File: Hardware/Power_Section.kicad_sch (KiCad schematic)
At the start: 39 parts, among them IC1 TPS54202HDDCR, Q1 SI2347DS-T1-GE3, U1 TLV743P, U2 TLV743P, U3 TLV743P, U4 TLV743P

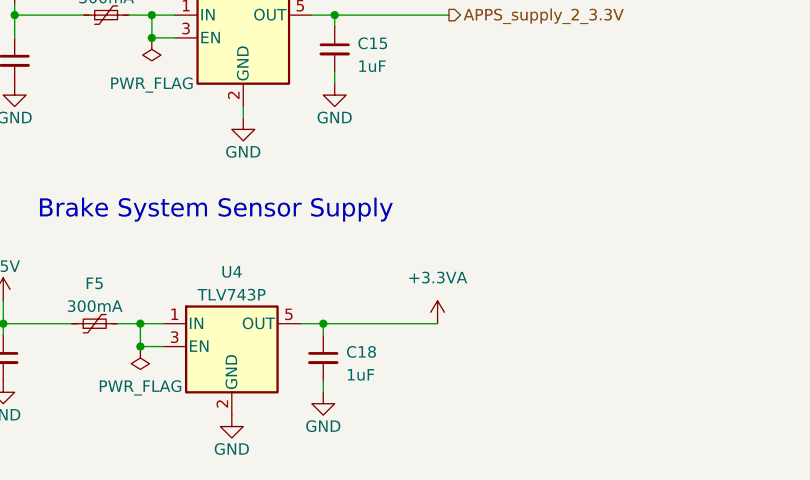
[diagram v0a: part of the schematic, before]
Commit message: Changes in CAN section
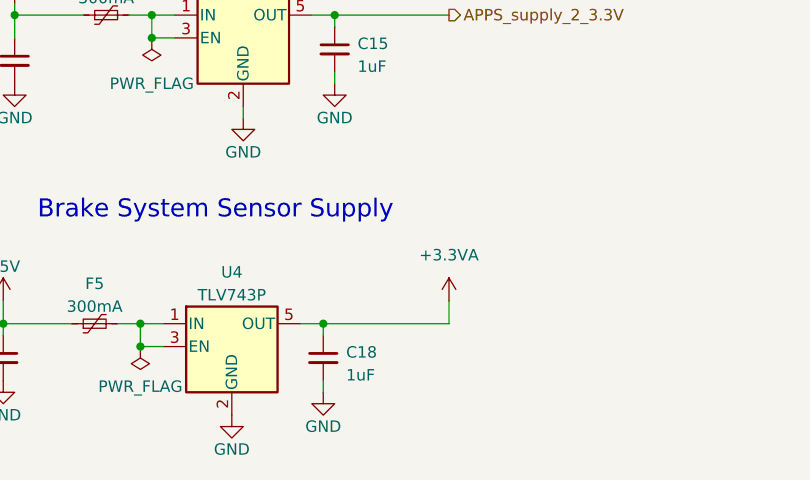
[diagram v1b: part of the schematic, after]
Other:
- title: (none) -> FrontBox
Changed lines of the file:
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@@
 	(generator_version "9.0")
 	(paper "A4")
+	(title_block
+		(title "FrontBox")
+	)
 	(text "APPS Potentiometer 2 supply"
 		(exclude_from_sim no)
@@
 	)
 	(junction
-		(at 64.77 172.72)
-		(diameter 0)
-		(color 0 0 0 0)
-	)
-	(junction
 		(at 245.11 59.69)
 		(diameter 0)
@@
 	)
 	(junction
+		(at 64.77 172.72)
+		(diameter 0)
+		(color 0 0 0 0)
+	)
+	(junction
 		(at 218.44 46.99)
 		(diameter 0)
@@
 	(wire
 		(pts
-			(xy 64.77 172.72) (xy 77.47 172.72)
-		)
-		(stroke
-			(width 0)
-			(type default)
-		)
-	)
-	(wire
-		(pts
 			(xy 25.4 72.39) (xy 25.4 73.66)
 		)
@@
 	(wire
 		(pts
+			(xy 64.77 172.72) (xy 78.74 172.72)
+		)
+		(stroke
+			(width 0)
+			(type default)
+		)
+	)
+	(wire
+		(pts
 			(xy 25.4 78.74) (xy 25.4 80.01)
 		)
@@
 	(wire
 		(pts
+			(xy 78.74 172.72) (xy 78.74 170.18)
+		)
+		(stroke
+			(width 0)
+			(type default)
+		)
+	)
+	(wire
+		(pts
 			(xy 245.11 46.99) (xy 255.27 46.99)
 		)
@@
 	(symbol
 		(lib_id "power:+3.3VA")
-		(at 77.47 172.72 0)
+		(at 78.74 170.18 0)
 		(unit 1)
 		(exclude_from_sim no)
@@
 		(dnp no)
 		(property "Reference" "#PWR036"
-			(at 77.47 176.53 0)
+			(at 78.74 173.99 0)
 			(effects
 				(font
@@
 		)
 		(property "Value" "+3.3VA"
-			(at 77.47 167.64 0)
+			(at 78.74 165.1 0)
 			(effects
 				(font
@@
 		)
 		(property "Footprint" ""
-			(at 77.47 172.72 0)
+			(at 78.74 170.18 0)
 			(effects
 				(font
@@
 		)
 		(property "Datasheet" ""
-			(at 77.47 172.72 0)
+			(at 78.74 170.18 0)
 			(effects
 				(font
@@
 		)
 		(property "Description" ""
-			(at 77.47 172.72 0)
+			(at 78.74 170.18 0)
 			(effects
 				(font

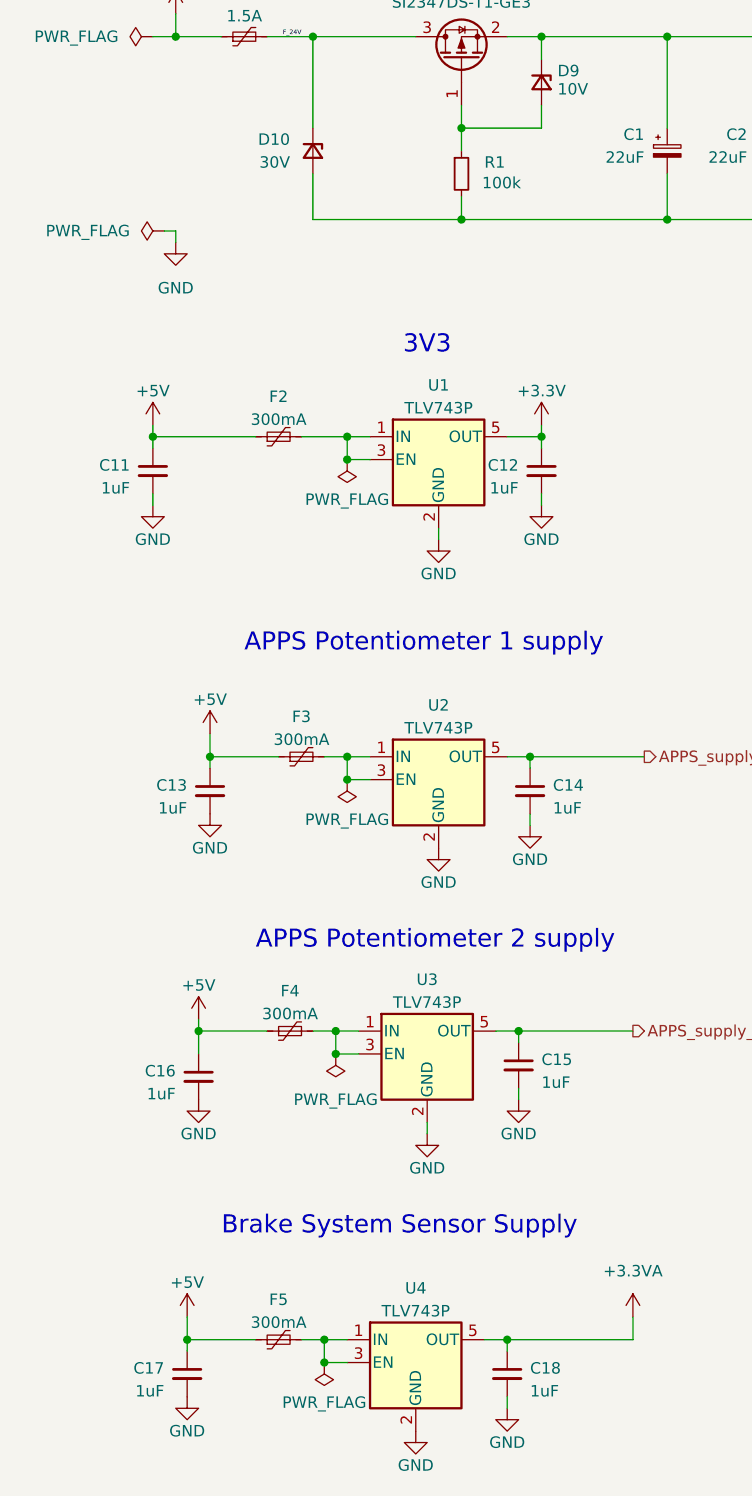
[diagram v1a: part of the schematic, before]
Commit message: BOM update
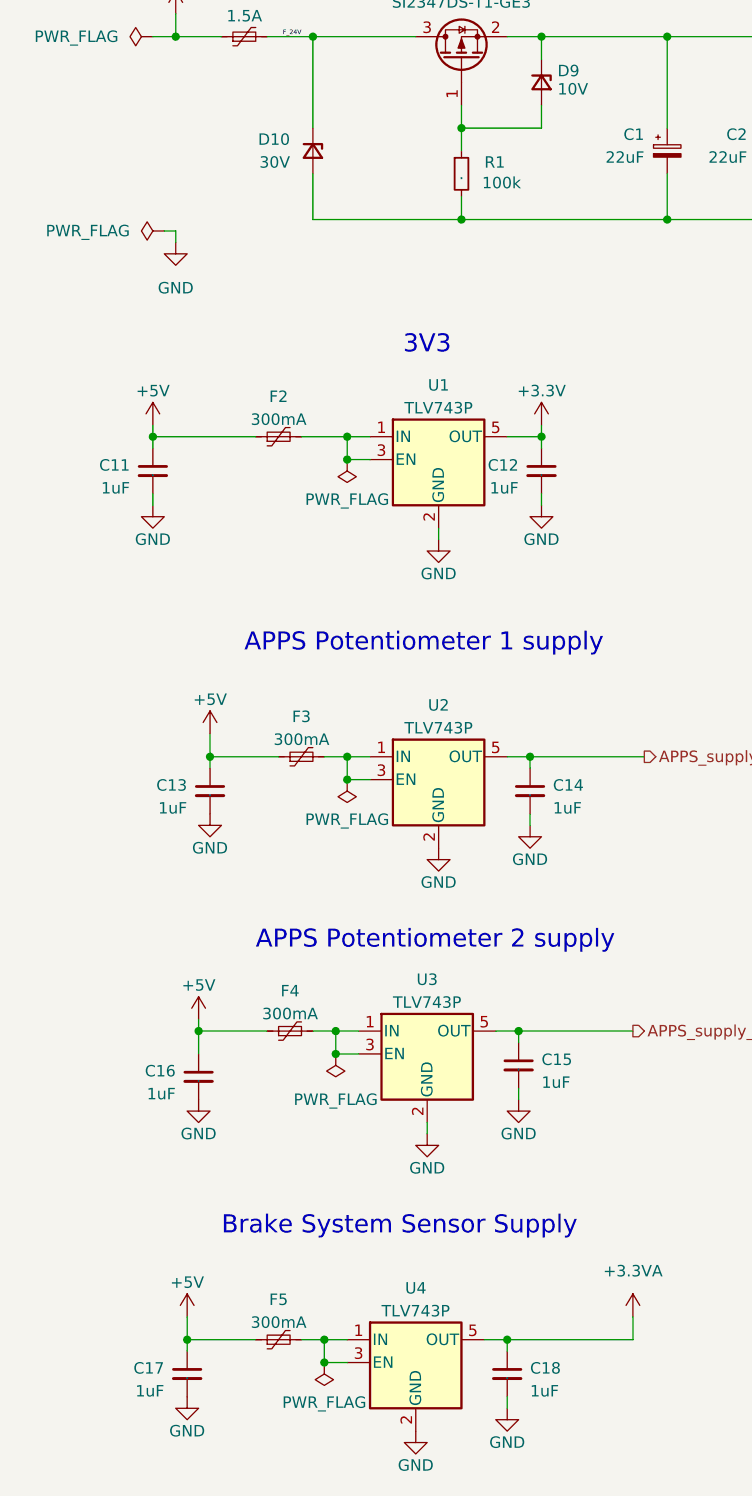
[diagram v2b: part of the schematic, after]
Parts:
- C11, C12, C13, C14, C15, C16, C17, C18, R1: Mouser Part Number (none) -> .
- F1: Mouser Part Number (none) -> 504-PTS181233V075
- F2, F3, F4, F5: Mouser Part Number (none) -> 603-SMD0603B010TF
- Q1: Mouser Part Number (none) -> 78-SI2347DS-T1-GE3
- U1, U2, U3, U4: Mouser Part Number (none) -> 595-TLV74333PDBVR
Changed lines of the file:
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@@
 			)
 		)
+		(property "Mouser Part Number" "."
+			(at 31.75 111.76 0)
+			(effects
+				(font
+					(size 1.27 1.27)
+				)
+			)
+		)
 		(pin "1"
 		)
@@
 			)
 		)
+		(property "Mouser Part Number" "78-SI2347DS-T1-GE3"
+			(at 59.69 30.48 0)
+			(effects
+				(font
+					(size 1.27 1.27)
+				)
+				(hide yes)
+			)
+		)
 		(pin "2"
 		)
@@
 			)
 		)
+		(property "Mouser Part Number" "504-PTS181233V075"
+			(at 35.56 27.94 0)
+			(effects
+				(font
+					(size 1.27 1.27)
+				)
+				(hide yes)
+			)
+		)
 		(pin "1"
 		)
@@
 			)
 		)
+		(property "Mouser Part Number" "."
+			(at 25.4 76.2 0)
+			(effects
+				(font
+					(size 1.27 1.27)
+				)
+			)
+		)
 		(pin "1"
 		)
@@
 			)
 		)
+		(property "Mouser Part Number" "603-SMD0603B010TF"
+			(at 39.37 172.72 0)
+			(effects
+				(font
+					(size 1.27 1.27)
+				)
+				(hide yes)
+			)
+		)
 		(pin "1"
 		)
@@
 			)
 		)
+		(property "Mouser Part Number" "603-SMD0603B010TF"
+			(at 40.64 138.43 0)
+			(effects
+				(font
+					(size 1.27 1.27)
+				)
+				(hide yes)
+			)
+		)
 		(pin "1"
 		)
@@
 			)
 		)
+		(property "Mouser Part Number" "."
+			(at 30.48 143.51 0)
+			(effects
+				(font
+					(size 1.27 1.27)
+				)
+			)
+		)
 		(pin "1"
 		)
@@
 			)
 		)
+		(property "Mouser Part Number" "595-TLV74333PDBVR"
+			(at 57.15 110.49 0)
+			(effects
+				(font
+					(size 1.27 1.27)
+				)
+				(hide yes)
+			)
+		)
 		(pin "1"
 		)
@@
 			)
 		)
+		(property "Mouser Part Number" "595-TLV74333PDBVR"
+			(at 57.15 74.93 0)
+			(effects
+				(font
+					(size 1.27 1.27)
+				)
+				(hide yes)
+			)
+		)
 		(pin "1"
 		)
@@
 			)
 		)
+		(property "Mouser Part Number" "."
+			(at 68.58 76.2 0)
+			(effects
+				(font
+					(size 1.27 1.27)
+				)
+			)
+		)
 		(pin "1"
 		)
@@
 			)
 		)
+		(property "Mouser Part Number" "."
+			(at 59.69 43.18 0)
+			(effects
+				(font
+					(size 1.27 1.27)
+				)
+			)
+		)
 		(pin "2"
 		)
@@
 			)
 		)
+		(property "Mouser Part Number" "."
+			(at 29.21 176.53 0)
+			(effects
+				(font
+					(size 1.27 1.27)
+				)
+			)
+		)
 		(pin "1"
 		)
@@
 			)
 		)
+		(property "Mouser Part Number" "595-TLV74333PDBVR"
+			(at 55.88 140.97 0)
+			(effects
+				(font
+					(size 1.27 1.27)
+				)
+				(hide yes)
+			)
+		)
 		(pin "1"
 		)
@@
 			)
 		)
+		(property "Mouser Part Number" "603-SMD0603B010TF"
+			(at 39.37 72.39 0)
+			(effects
+				(font
+					(size 1.27 1.27)
+				)
+				(hide yes)
+			)
+		)
 		(pin "1"
 		)
@@
 			)
 		)
+		(property "Mouser Part Number" "."
+			(at 64.77 176.53 0)
+			(effects
+				(font
+					(size 1.27 1.27)
+				)
+			)
+		)
 		(pin "1"
 		)
@@
 			)
 		)
+		(property "Mouser Part Number" "."
+			(at 66.04 142.24 0)
+			(effects
+				(font
+					(size 1.27 1.27)
+				)
+			)
+		)
 		(pin "1"
 		)
@@
 			)
 		)
+		(property "Mouser Part Number" "603-SMD0603B010TF"
+			(at 41.91 107.95 0)
+			(effects
+				(font
+					(size 1.27 1.27)
+				)
+				(hide yes)
+			)
+		)
 		(pin "1"
 		)
@@
 			)
 		)
+		(property "Mouser Part Number" "."
+			(at 67.31 111.76 0)
+			(effects
+				(font
+					(size 1.27 1.27)
+				)
+			)
+		)
 		(pin "1"
 		)
@@
 			(at 54.61 175.26 0)
 			(effects
+				(font
+					(size 1.27 1.27)
+				)
+				(hide yes)
+			)
+		)
+		(property "Mouser Part Number" "595-TLV74333PDBVR"
+			(at 54.61 175.26 0)
+			(effects
